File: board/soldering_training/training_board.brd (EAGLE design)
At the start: 68.6 x 53.4 mm, 24 parts, among them J1 MAIN_PWR, Q1 ARDUINOR3-NOIOREF-NOTEXT, Q2 DMN2056U, SW2 PTS645, U1 DRV8871HSOP-8

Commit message: Renamed SW2 to SW1
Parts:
- renumbered SW2 to SW1
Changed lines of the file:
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@@
 <drawing>
 <settings>
-<setting alwaysvectorfont="yes"/>
+<setting alwaysvectorfont="no"/>
 <setting verticaltext="up"/>
 </settings>
-<grid distance="50" unitdist="mil" unit="mm" style="lines" multiple="1" display="no" altdistance="5" altunitdist="mil" altunit="mm"/>
+<grid distance="50" unitdist="mil" unit="mil" style="lines" multiple="1" display="no" altdistance="5" altunitdist="mil" altunit="mil"/>
 <layers>
 <layer number="1" name="Top" color="4" fill="1" visible="yes" active="yes"/>
@@
 </element>
 <element name="J1" library="RoboJackets-Connectors" package="PJ-037A" value="MAIN_PWR" x="3.43" y="26.25" smashed="yes"/>
-<element name="SW2" library="RoboJackets-Switches" package="PTS645" value="PTS645" x="36.5" y="12.15" smashed="yes">
+<element name="SW1" library="RoboJackets-Switches" package="PTS645" value="PTS645" x="36.5" y="12.15" smashed="yes">
 <attribute name="FUNCTION" value="RESET" x="36.5" y="12.15" size="1.778" layer="27" font="vector" display="off"/>
 </element>
@@
 <contactref element="J1" pad="P$1"/>
 <contactref element="Q1" pad="GND1"/>
-<contactref element="SW2" pad="2"/>
-<contactref element="SW2" pad="1"/>
+<contactref element="SW1" pad="2"/>
+<contactref element="SW1" pad="1"/>
 <contactref element="LED3" pad="C"/>
 <contactref element="LED4" pad="C"/>
@@
 <signal name="RESET">
 <contactref element="Q1" pad="RESET"/>
-<contactref element="SW2" pad="3"/>
-<contactref element="SW2" pad="4"/>
+<contactref element="SW1" pad="3"/>
+<contactref element="SW1" pad="4"/>
 <contactref element="R4" pad="1"/>
 <contactref element="C3" pad="1"/>

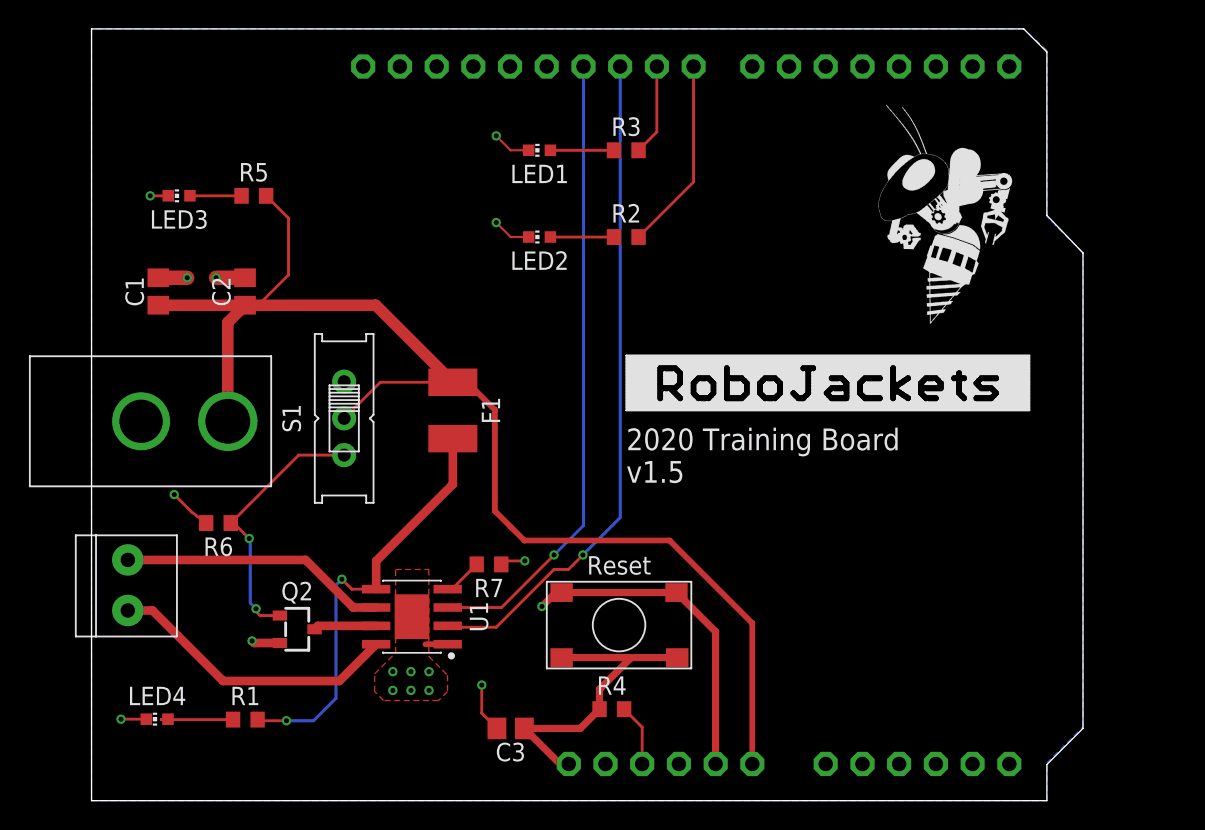
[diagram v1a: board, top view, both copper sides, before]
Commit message: Fixed minor issues and made roboBuzz bigger
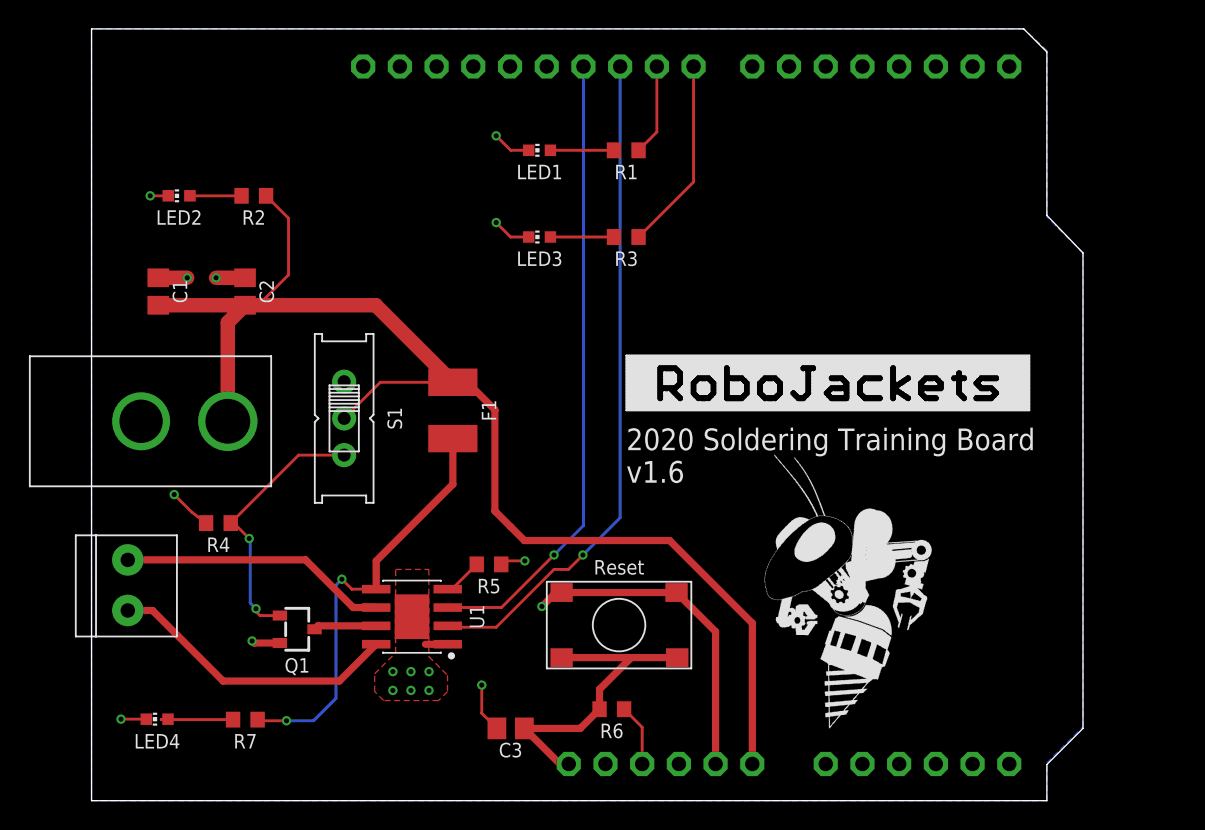
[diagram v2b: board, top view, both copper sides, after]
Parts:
- removed U$4: (no value), RoboJackets-Aesthetics:ROBOBUZZ_0.8X
- added U$2: (no value), RoboJackets-Aesthetics:ROBOBUZZ_1.0X
- C3: value 0.1uF 6V -> 0.1uF 16V
- LED2: value ORANGE -> GREEN
- LED3: value GREEN -> ORANGE
- Q1: value ARDUINOR3-NOIOREF-NOTEXT -> DMN2056U; device adafruit:ARDUINOR3-NOTEXT-NOIOREF -> RoboJackets-Discrete:SOT-23-3
- Q2: value DMN2056U -> ARDUINOR3-NOIOREF-NOTEXT; device RoboJackets-Discrete:SOT-23-3 -> adafruit:ARDUINOR3-NOTEXT-NOIOREF
- R1: value 2.4K -> 1K
- R2: value 1K -> 2.4K
- R5: value 2.4K -> 120K
- R7: value 120K -> 2.4K
- moved R1 47.4 mm to (37.0, 45.0)
- moved R5 30.2 mm to (27.5, 16.4)
- moved R4 30.1 mm to (8.78, 19.2), turned to 180 degrees
- moved R6 30.1 mm to (36.0, 6.33), turned to 0 degrees
- moved R2 25.9 mm to (11.2, 41.9)
- moved LED2 25.1 mm to (6.06, 41.9)
- moved LED3 25.1 mm to (31.0, 39.0)
- moved R7 20.0 mm to (10.6, 5.61)
- moved Q1 18.5 mm to (14.2, 11.9), turned to 270 degrees
- moved Q2 18.5 mm to (0.00, 0.00), turned to 0 degrees
- moved R3 6.00 mm to (37.0, 39.0)
- renumbered U$3 to U$1
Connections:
- removed net N$16 (its old number): LED3.A, R5.1
- new net N$15: LED3.A, R3.1
- net +12V: now also Q2.VIN, R2.2; no longer Q1.VIN, R5.2
- net +5V: now also Q2.5V, R6.2; no longer Q1.5V, R4.2
- net 3V: now also Q2.3V; no longer Q1.3V
- net GND: now also Q1.2, Q2.GND, Q2.GND1, Q2.GND2, R4.2, R5.2; no longer Q1.GND, Q1.GND1, Q1.GND2, Q2.2, R6.2, R7.2
- net M1_FWD: now also Q2.D10; no longer Q1.D10
- net M1_REV: now also Q2.D11; no longer Q1.D11
- net N$1: now also R7.2; no longer R1.2
- net N$10: now also Q2.D9, R1.2; no longer Q1.D9, R3.2
- net N$11: now also Q2.D8, R3.2; no longer Q1.D8, R2.2
- net N$14: now also R1.1; no longer R3.1
- net N$3: now also Q1.3; no longer Q2.3
- net N$5: now also Q1.1, R4.1; no longer Q2.1, R6.1
- net N$6: now also R5.1; no longer R7.1
- net N$8: now also R7.1; no longer R1.1
- net RESET: now also Q2.RESET, R6.1; no longer Q1.RESET, R4.1
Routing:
- net N$15: track 0.00 -> 4.40 mm
- net N$16 (its old number): track 3.57 -> 0.00 mm
- net N$16: track 4.40 -> 3.57 mm
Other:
- board text added: "2020 Soldering Training Board v1.6"
- board text removed: "2020 Training Board v1.5"
